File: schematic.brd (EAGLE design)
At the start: 83.5 x 80 mm, 48 parts, among them U1 FT232RL-BASICSSOP

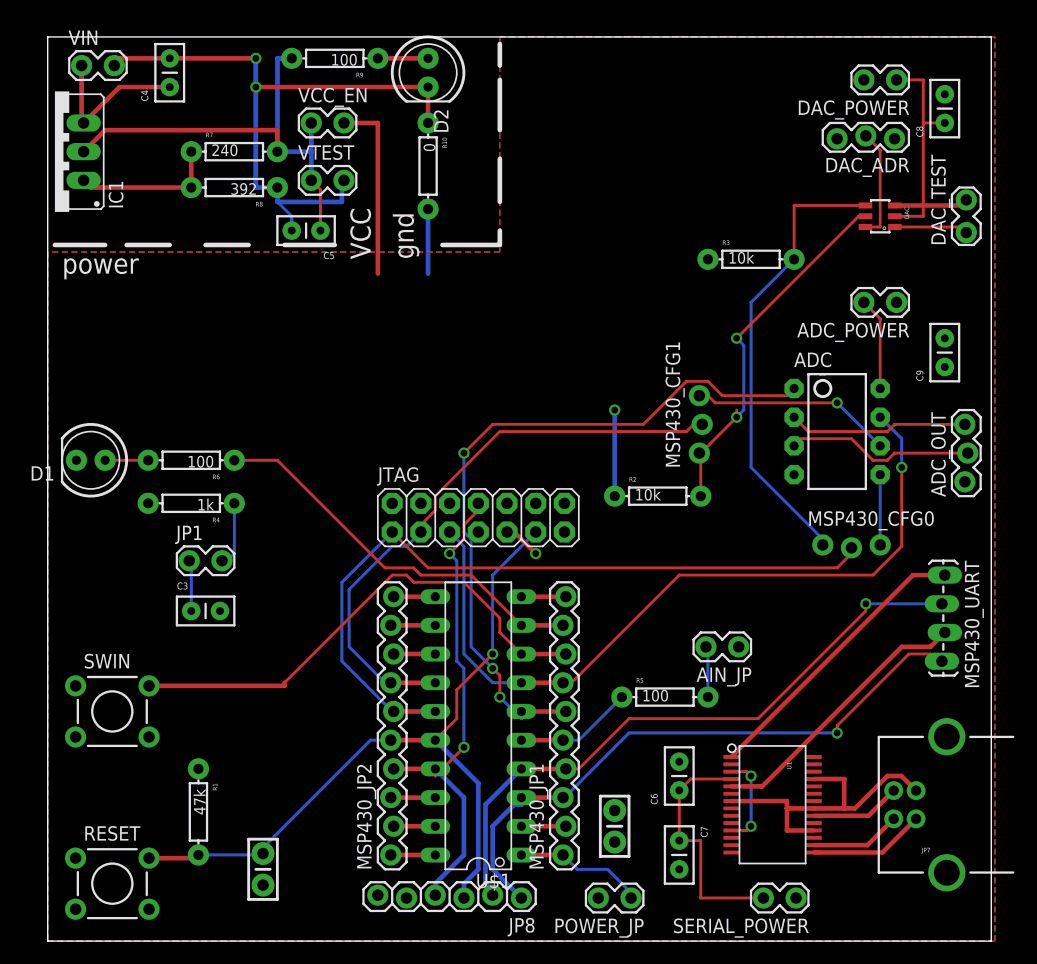
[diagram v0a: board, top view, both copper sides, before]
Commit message: finishing up layout
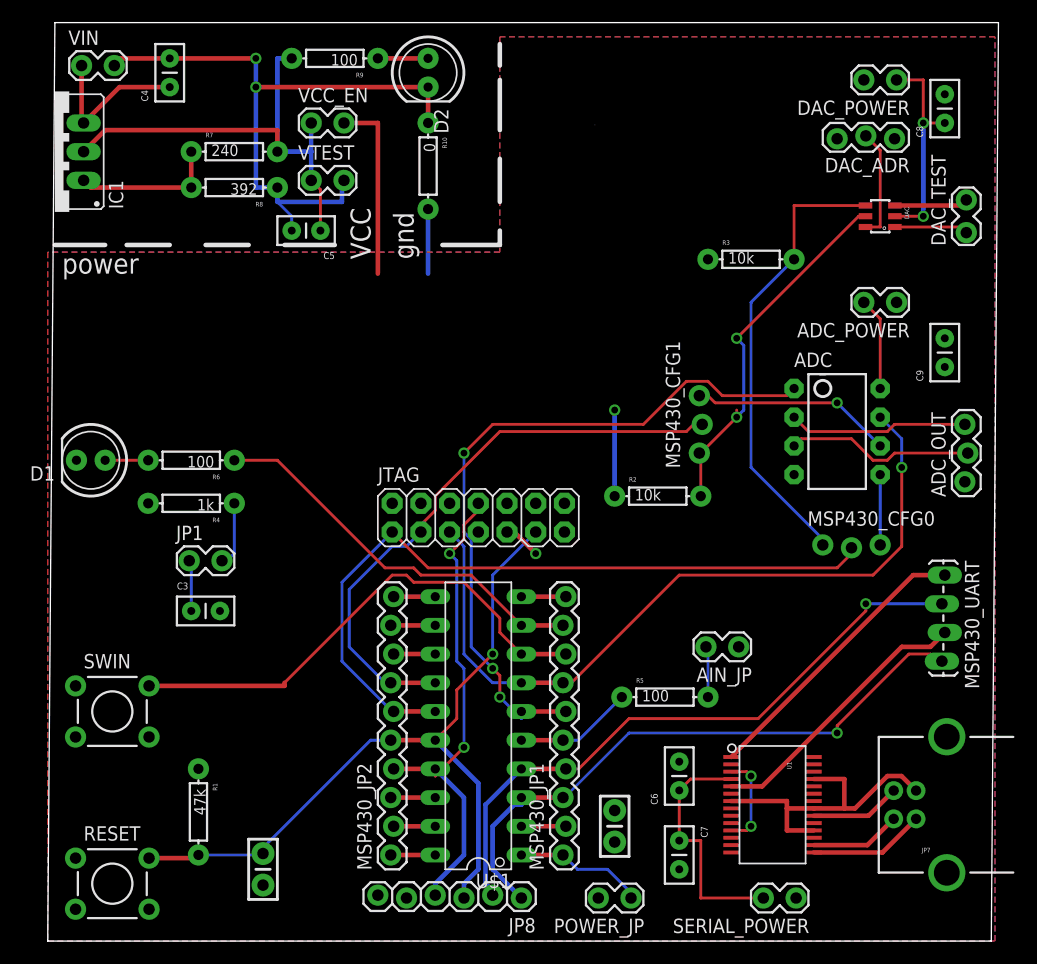
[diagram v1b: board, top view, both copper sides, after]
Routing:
- net N$14: vias 0 -> 2
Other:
- board size 83.5 x 80 mm -> 84.1 x 81.3 mm
- board text added: "/Users/Alex/Desktop/logo.bmp"
